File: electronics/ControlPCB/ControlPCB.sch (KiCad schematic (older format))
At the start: 70 parts, among them P1 CONN_02X03, P2 CONN_02X03, P3 CONN_02X03, P4 CONN_02X03, P5 CONN_02X03, P6 CONN_02X03, P7 CONN_02X03, P8 CONN_02X03, U1 POLOLU_A4988, U2 POLOLU_A4988, U3 POLOLU_A4988, U4 POLOLU_A4988, U5 POLOLU_A4988, U6 POLOLU_A4988, U7 POLOLU_A4988, U8 POLOLU_A4988

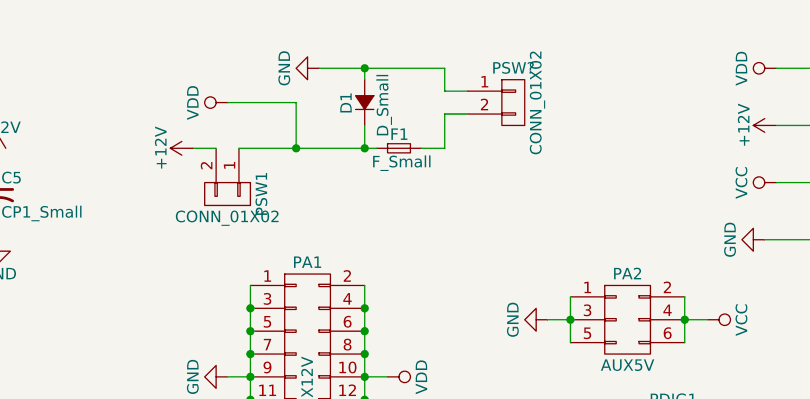
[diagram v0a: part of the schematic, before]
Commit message: Gerber files uploaded
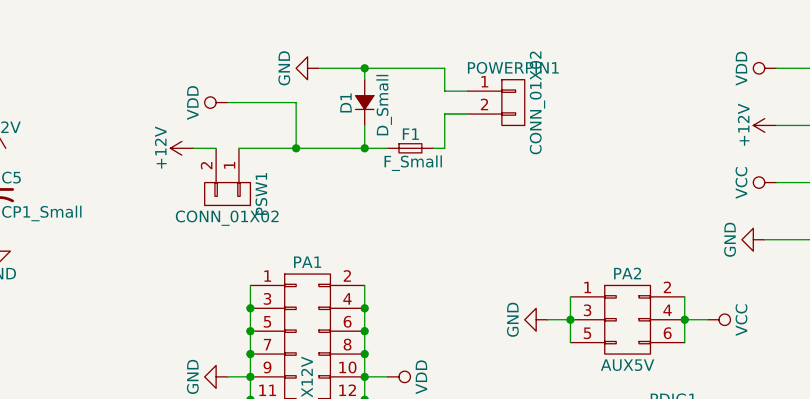
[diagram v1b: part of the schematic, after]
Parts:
- gave numbers to parts that had none: 1
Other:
- moved on the sheet: F1
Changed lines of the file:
@@
 L F_Small F1
 U 1 1 58303340
-P 8900 1150
-F 0 "F1" H 8860 1210 50  0000 L CNN
-F 1 "F_Small" H 8780 1090 50  0000 L CNN
-F 2 "Fuse_Holders_and_Fuses:BladeFuse-CarType" H 8900 1150 50  0001 C CNN
-F 3 "" H 8900 1150 50  0000 C CNN
-	1    8900 1150
+P 8950 1150
+F 0 "F1" H 8910 1210 50  0000 L CNN
+F 1 "F_Small" H 8830 1090 50  0000 L CNN
+F 2 "Fuse_Holders_and_Fuses:BladeFuse-CarType" H 8950 1150 50  0001 C CNN
+F 3 "" H 8950 1150 50  0000 C CNN
+	1    8950 1150
 	1    0    0    -1
 $EndComp
@@
 	9100 1000 9100 1150
 Wire Wire Line
-	9100 1150 9000 1150
-Wire Wire Line
 	8750 1150 8750 1050
 Connection ~ 8750 1150
@@
 Connection ~ 8750 800
 Wire Wire Line
-	8200 1150 8800 1150
+	8200 1150 8850 1150
 Wire Wire Line
 	8100 1150 8000 1150
@@
 	9850 3250 9800 3250
 $Comp
-L CONN_01X02 PSW?
+L CONN_01X02 POWERPIN1
 U 1 1 58406269
 P 9400 950
-F 0 "PSW?" H 9400 1100 50  0000 C CNN
+F 0 "POWERPIN1" H 9400 1100 50  0000 C CNN
 F 1 "CONN_01X02" V 9500 950 50  0000 C CNN
 F 2 "Pin_Headers:Pin_Header_Straight_1x02" H 9400 950 50  0001 C CNN
@@
 Wire Wire Line
 	9200 1000 9100 1000
+Wire Wire Line
+	9100 1150 9050 1150
 $EndSCHEMATC
